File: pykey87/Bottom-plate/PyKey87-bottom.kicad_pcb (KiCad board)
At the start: 2 copper layers, 353 x 120 mm, 10 parts

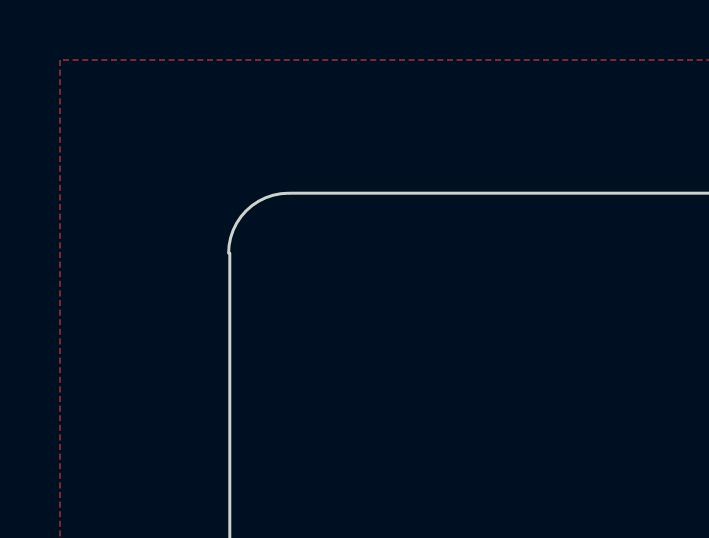
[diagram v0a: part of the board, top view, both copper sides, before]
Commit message: Misc fixes to schematic, PCB, and plates
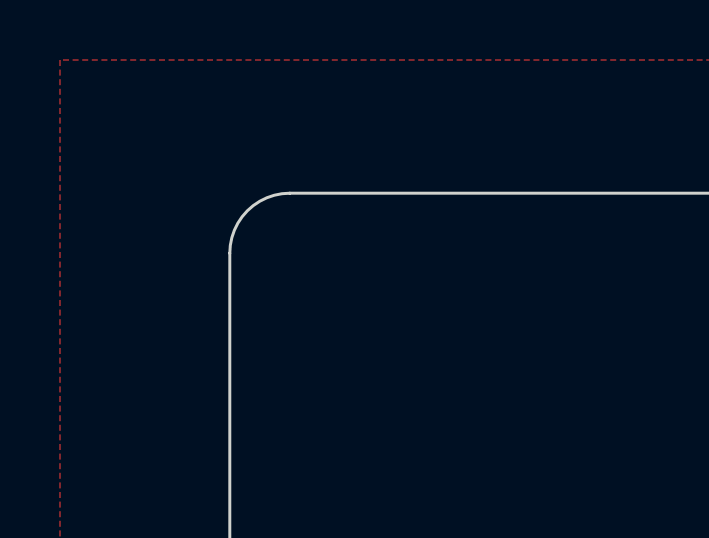
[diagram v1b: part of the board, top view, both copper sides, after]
